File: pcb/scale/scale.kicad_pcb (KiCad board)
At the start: 2 copper layers, 103.8 x 47.9 mm, 89 parts, among them J1 USB_C_Receptacle_USB2.0, J2 Conn_01x07, J3 Conn_01x04, SW1 SW_Push, SW10 SW_Push, SW11 SW_Push, SW12 SW_Push, SW13 SW_Push, SW14 SW_Push, SW15 SW_Push, SW16 SW_Push, SW17 SW_Push, SW18 SW_Push, SW2 SW_Push, SW3 SW_Push, SW4 SW_Push, SW5 SW_Push, SW6 SW_Push, SW7 SW_Push, SW8 SW_Push, SW9 SW_Push, U1 TP4065, U2 SPX3819M5-L-3-3, U3 STM32F103C8Tx, U4 CAT3200-5, U5 CS1237, U6 DS18B20, Y1 Crystal_GND24_Small, Y2 Crystal_Small

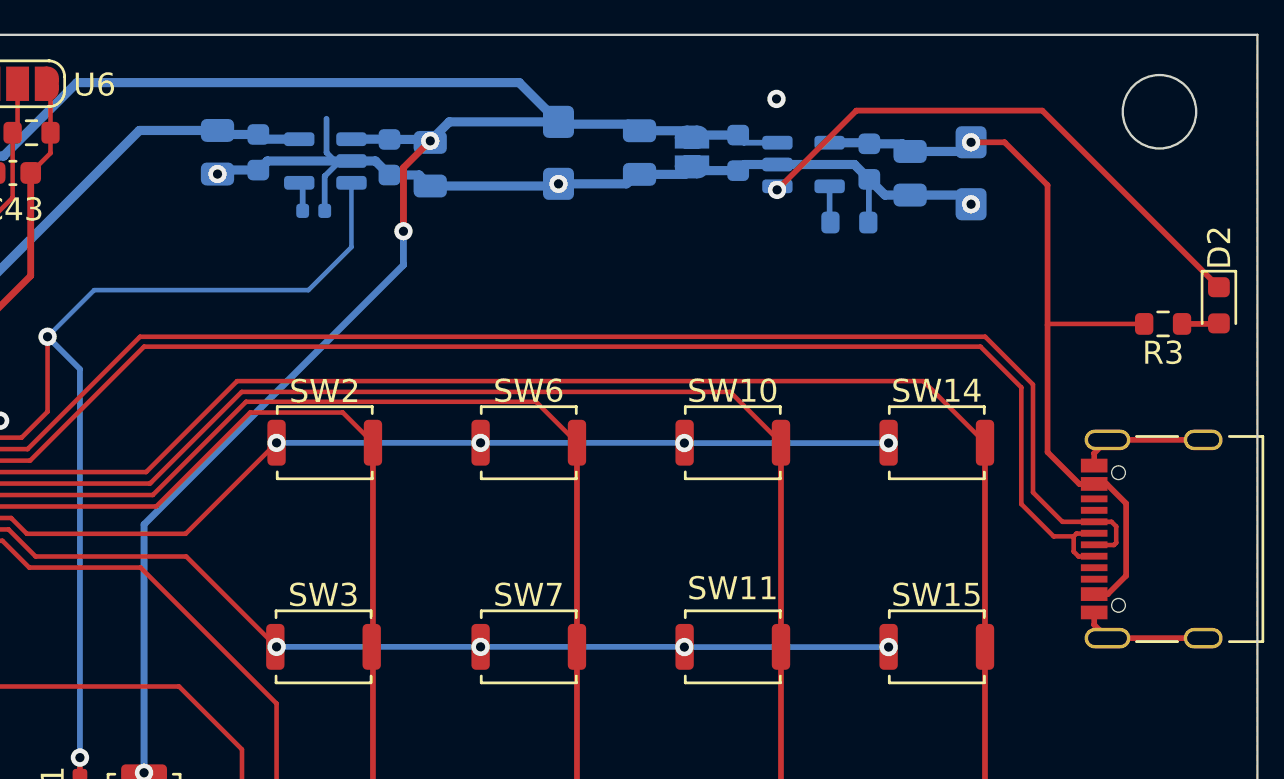
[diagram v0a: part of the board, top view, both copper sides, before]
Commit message: 微调布线
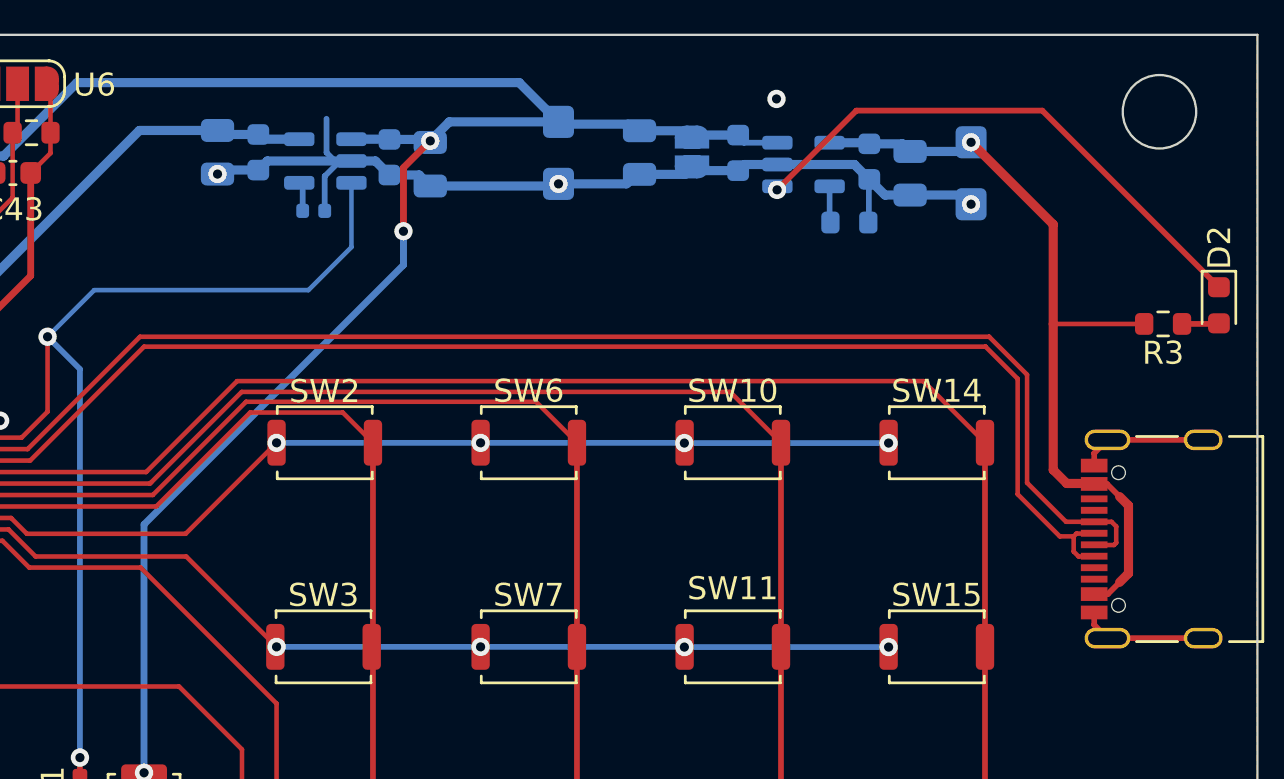
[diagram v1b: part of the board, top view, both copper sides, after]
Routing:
- net VBUS: track 35.6 -> 34.6 mm
- net GND: track 166.4 -> 165.9 mm
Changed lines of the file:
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@@
   (segment (start 73.787 61.008) (end 73.962 60.833) (width 0.4) (layer "B.Cu") (net 2))
   (segment (start 73.787 62.611) (end 73.787 61.008) (width 0.4) (layer "B.Cu") (net 2))
-  (segment (start 165.9335 76.7095) (end 166.315 77.091) (width 0.25) (layer "B.Cu") (net 2))
   (segment (start 93.151 59.5592) (end 93.0148 59.423) (width 0.4) (layer "B.Cu") (net 2))
   (segment (start 133.3699 56.2988) (end 129.7054 56.2988) (width 0.4) (layer "B.Cu") (net 2))
@@
   (segment (start 106.2736 66.4464) (end 107.2616 66.4464) (width 0.25) (layer "F.Cu") (net 11))
   (segment (start 107.2616 66.4464) (end 107.2896 66.4184) (width 0.25) (layer "F.Cu") (net 11))
+  (segment (start 115.7955 69.354) (end 119.368 69.354) (width 0.2) (layer "F.Cu") (net 12))
   (segment (start 164.9644 72.5334) (end 165.735 72.5334) (width 0.2) (layer "F.Cu") (net 12))
   (segment (start 165.735 73.5334) (end 165.058 73.5334) (width 0.2) (layer "F.Cu") (net 12))
   (segment (start 164.8414 73.3168) (end 164.8414 72.6564) (width 0.2) (layer "F.Cu") (net 12))
   (segment (start 165.058 73.5334) (end 164.8414 73.3168) (width 0.2) (layer "F.Cu") (net 12))
-  (segment (start 162.56 71.247) (end 163.9694 72.6564) (width 0.2) (layer "F.Cu") (net 12))
+  (segment (start 162.4 65.789) (end 162.4 70.819) (width 0.2) (layer "F.Cu") (net 12))
+  (segment (start 160.999 64.388) (end 162.4 65.789) (width 0.2) (layer "F.Cu") (net 12))
+  (segment (start 164.8414 72.6564) (end 164.9644 72.5334) (width 0.2) (layer "F.Cu") (net 12))
+  (segment (start 164.8404 72.6554) (end 164.8414 72.6564) (width 0.2) (layer "F.Cu") (net 12))
   (segment (start 119.368 69.354) (end 124.333 64.389) (width 0.2) (layer "F.Cu") (net 12))
-  (segment (start 115.7955 69.354) (end 119.368 69.354) (width 0.2) (layer "F.Cu") (net 12))
-  (segment (start 163.9694 72.6564) (end 164.8414 72.6564) (width 0.2) (layer "F.Cu") (net 12))
-  (segment (start 162.56 66.167) (end 162.56 71.247) (width 0.2) (layer "F.Cu") (net 12))
-  (segment (start 160.782 64.389) (end 162.56 66.167) (width 0.2) (layer "F.Cu") (net 12))
-  (segment (start 124.333 64.389) (end 160.782 64.389) (width 0.2) (layer "F.Cu") (net 12))
-  (segment (start 164.8414 72.6564) (end 164.9644 72.5334) (width 0.2) (layer "F.Cu") (net 12))
-  (segment (start 164.35 72.021) (end 165.735 72.021) (width 0.2) (layer "F.Cu") (net 13))
+  (segment (start 162.4 70.819) (end 164.2364 72.6554) (width 0.2) (layer "F.Cu") (net 12))
+  (segment (start 164.2364 72.6554) (end 164.8404 72.6554) (width 0.2) (layer "F.Cu") (net 12))
+  (segment (start 124.333 64.389) (end 160.998 64.389) (width 0.2) (layer "F.Cu") (net 12))
+  (segment (start 160.998 64.389) (end 160.999 64.388) (width 0.2) (layer "F.Cu") (net 12))
+  (segment (start 161.1572 63.9562) (end 162.81 65.609) (width 0.2) (layer "F.Cu") (net 13))
+  (segment (start 166.598 73.0334) (end 165.735 73.0334) (width 0.2) (layer "F.Cu") (net 13))
+  (segment (start 165.734 72.02) (end 165.735 72.021) (width 0.2) (layer "F.Cu") (net 13))
+  (segment (start 166.6956 72.2246) (end 166.6956 72.9358) (width 0.2) (layer "F.Cu") (net 13))
+  (segment (start 119.2584 68.854) (end 124.1552 63.9572) (width 0.2) (layer "F.Cu") (net 13))
+  (segment (start 166.492 72.021) (end 166.6956 72.2246) (width 0.2) (layer "F.Cu") (net 13))
+  (segment (start 162.81 65.609) (end 162.81 70.32) (width 0.2) (layer "F.Cu") (net 13))
+  (segment (start 124.1552 63.9572) (end 161.1562 63.9572) (width 0.2) (layer "F.Cu") (net 13))
+  (segment (start 162.81 70.32) (end 164.51 72.02) (width 0.2) (layer "F.Cu") (net 13))
+  (segment (start 164.51 72.02) (end 165.734 72.02) (width 0.2) (layer "F.Cu") (net 13))
+  (segment (start 161.1562 63.9572) (end 161.1572 63.9562) (width 0.2) (layer "F.Cu") (net 13))
   (segment (start 115.7955 68.854) (end 119.2584 68.854) (width 0.2) (layer "F.Cu") (net 13))
-  (segment (start 166.598 73.0334) (end 165.735 73.0334) (width 0.2) (layer "F.Cu") (net 13))
-  (segment (start 166.6956 72.2246) (end 166.6956 72.9358) (width 0.2) (layer "F.Cu") (net 13))
-  (segment (start 160.9852 63.9572) (end 163.068 66.04) (width 0.2) (layer "F.Cu") (net 13))
-  (segment (start 166.492 72.021) (end 166.6956 72.2246) (width 0.2) (layer "F.Cu") (net 13))
-  (segment (start 163.068 70.739) (end 164.35 72.021) (width 0.2) (layer "F.Cu") (net 13))
-  (segment (start 119.2584 68.854) (end 124.1552 63.9572) (width 0.2) (layer "F.Cu") (net 13))
-  (segment (start 163.068 66.04) (end 163.068 70.739) (width 0.2) (layer "F.Cu") (net 13))
-  (segment (start 124.1552 63.9572) (end 160.9852 63.9572) (width 0.2) (layer "F.Cu") (net 13))
   (segment (start 166.6956 72.9358) (end 166.598 73.0334) (width 0.2) (layer "F.Cu") (net 13))
   (segment (start 165.735 72.021) (end 166.492 72.021) (width 0.2) (layer "F.Cu") (net 13))
@@
   (segment (start 130.107 95.25) (end 138.997 95.25) (width 0.25) (layer "B.Cu") (net 43))
   (segment (start 138.997 95.25) (end 147.887 95.25) (width 0.25) (layer "B.Cu") (net 43))
-  (segment (start 161.8326 55.4828) (end 160.37115 55.4828) (width 0.25) (layer "F.Cu") (net 44))
-  (segment (start 163.703 63.4492) (end 163.703 57.3532) (width 0.25) (layer "F.Cu") (net 44))
-  (segment (start 163.703 57.3532) (end 161.8326 55.4828) (width 0.25) (layer "F.Cu") (net 44))
-  (segment (start 165.735 70.371) (end 165.0876 70.371) (width 0.25) (layer "F.Cu") (net 44))
-  (segment (start 166.3276 75.171) (end 167.1274 74.3712) (width 0.25) (layer "F.Cu") (net 44))
-  (segment (start 167.1274 71.2216) (end 167.1274 74.3712) (width 0.25) (layer "F.Cu") (net 44))
-  (segment (start 167.9133 63.3984) (end 163.7538 63.3984) (width 0.2) (layer "F.Cu") (net 44))
-  (segment (start 166.2768 70.371) (end 167.1274 71.2216) (width 0.25) (layer "F.Cu") (net 44))
-  (segment (start 163.703 68.9864) (end 163.703 63.4492) (width 0.25) (layer "F.Cu") (net 44))
-  (segment (start 163.7538 63.3984) (end 163.703 63.4492) (width 0.2) (layer "F.Cu") (net 44))
-  (segment (start 165.735 75.171) (end 166.3276 75.171) (width 0.25) (layer "F.Cu") (net 44))
-  (segment (start 165.735 70.371) (end 166.2768 70.371) (width 0.25) (layer "F.Cu") (net 44))
-  (segment (start 165.0876 70.371) (end 163.703 68.9864) (width 0.25) (layer "F.Cu") (net 44))
+  (segment (start 167.23 71.31) (end 167.23 74.27) (width 0.4) (layer "F.Cu") (net 44))
+  (segment (start 167.9133 63.3984) (end 167.9117 63.4) (width 0.2) (layer "F.Cu") (net 44))
+  (segment (start 166.329 75.171) (end 166.84 74.66) (width 0.25) (layer "F.Cu") (net 44))
+  (segment (start 167.23 74.27) (end 166.84 74.66) (width 0.4) (layer "F.Cu") (net 44))
+  (segment (start 163.95 69.76) (end 163.95 63.4) (width 0.4) (layer "F.Cu") (net 44))
+  (segment (start 166.84 70.92) (end 167.23 71.31) (width 0.4) (layer "F.Cu") (net 44))
+  (segment (start 165.735 70.371) (end 166.291 70.371) (width 0.25) (layer "F.Cu") (net 44))
+  (segment (start 165.4545 70.3505) (end 164.5405 70.3505) (width 0.4) (layer "F.Cu") (net 44))
+  (segment (start 163.95 59.06165) (end 160.37115 55.4828) (width 0.4) (layer "F.Cu") (net 44))
+  (segment (start 163.95 63.4) (end 163.95 59.06165) (width 0.4) (layer "F.Cu") (net 44))
+  (segment (start 165.735 75.171) (end 166.329 75.171) (width 0.25) (layer "F.Cu") (net 44))
+  (segment (start 164.5405 70.3505) (end 163.95 69.76) (width 0.4) (layer "F.Cu") (net 44))
+  (segment (start 167.9117 63.4) (end 163.95 63.4) (width 0.2) (layer "F.Cu") (net 44))
+  (segment (start 166.291 70.371) (end 166.84 70.92) (width 0.25) (layer "F.Cu") (net 44))
   (via (at 160.37115 55.4828) (size 0.8) (drill 0.4) (layers "F.Cu" "B.Cu") (net 44))
   (segment (start 155.9359 55.5498) (end 157.3809 55.5498) (width 0.4) (layer "B.Cu") (net 44))
